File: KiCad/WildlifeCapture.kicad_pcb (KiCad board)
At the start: 2 copper layers, 105 x 100 mm, 15 parts, among them P1 USB_A, P2 GPS, SW1 A, SW2 LEADSW, U1 IM920_interplan, U3 STM32F103C8T6MinimumDevelopBo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, U4 RASPBERRYPI_GPIO_40

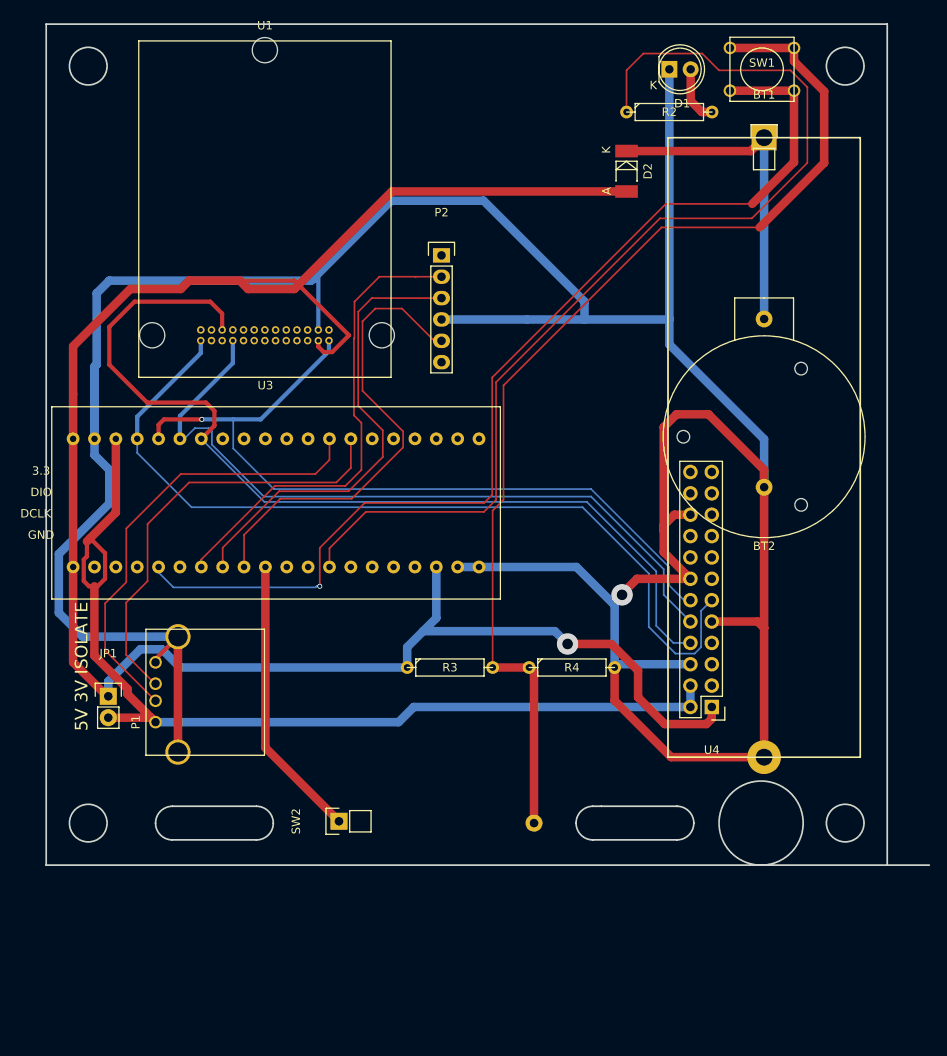
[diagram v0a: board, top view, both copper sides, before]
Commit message: Change to Take 2
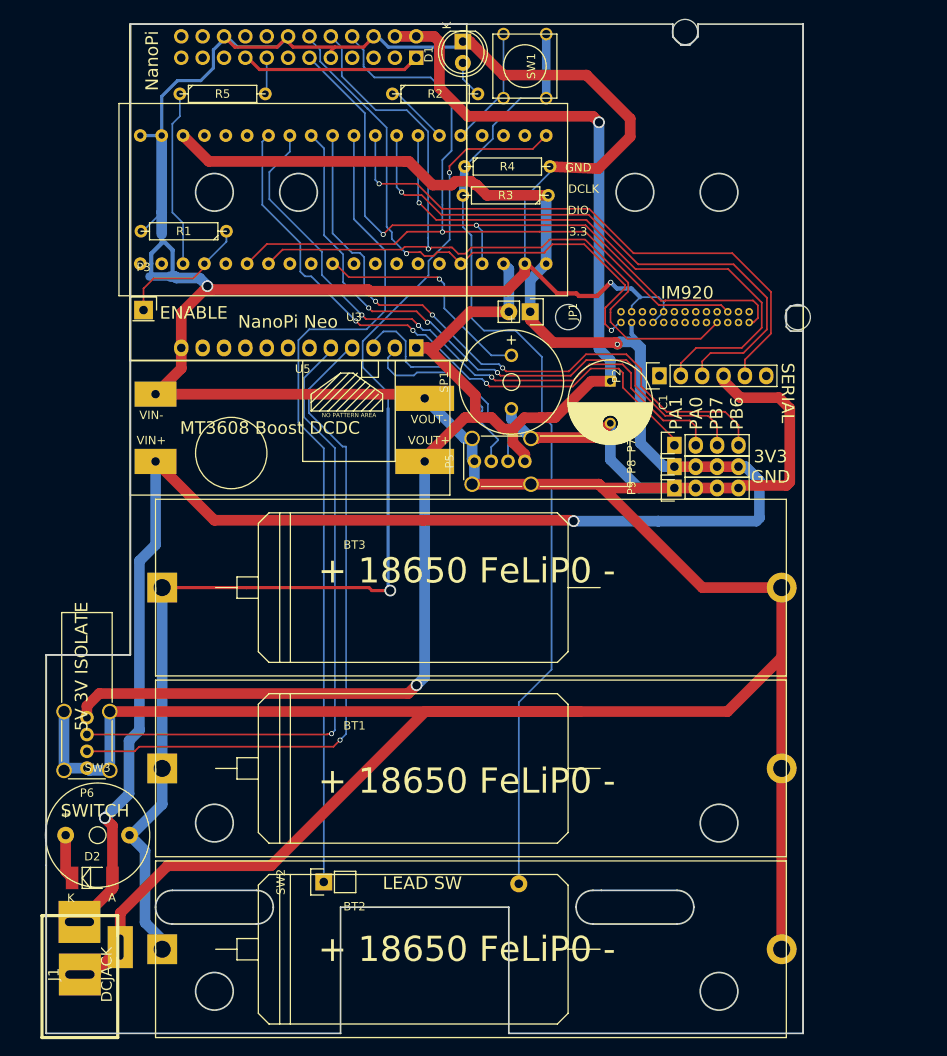
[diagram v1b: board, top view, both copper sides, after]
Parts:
- removed P1: USB_A, Connect:USB_A
- added BT3: Battery, library:18650BatteryCase, F.Cu at (134.1, 103.2)
- added C1: CP1, Capacitors_ThroughHole:C_Radial_D10_L13_P5, F.Cu at (158.2, 78.7)
- added J1: DCJACK, library:DCJACK, F.Cu at (95.1, 149.2)
- added P3: EN, Pin_Headers:Pin_Header_Straight_1x01, F.Cu at (102.7, 70.2)
- added P4: NanoPi_USB/Audio/IR, Pin_Headers:Pin_Header_Straight_1x12, B.Cu at (135.1, 74.7)
- added P5: USB_A, Connect:USB_A_Vertical, F.Cu at (148.0, 88.2)
- added P6: USB_A, Connect:USB_A_Vertical, F.Cu at (95.9, 118.7)
- added P7: SERVICE, Pin_Headers:Pin_Header_Straight_1x04, F.Cu at (165.8, 86.3)
- added P8: VCC, Pin_Headers:Pin_Header_Straight_1x04, F.Cu at (165.8, 88.9)
- added P9: GND, Pin_Headers:Pin_Header_Straight_1x04, F.Cu at (165.8, 91.4)
- added R1: R, Discret:R4, F.Cu at (107.4, 60.9)
- added R5: R, Discret:R4, F.Cu at (112.1, 44.5)
- added SP1: SPEAKER, Buzzers_Beepers:MagneticBuzzer_ProSignal_ABT-410-RC, F.Cu at (146.4, 82.0)
- added SW3: SWITCH_INV, Buzzers_Beepers:Buzzer_12x9.5RM7.6, F.Cu at (97.2, 132.7)
- added U5: MT3608, library:MT3608, F.Cu at (120.1, 84.2)
- BT1: footprint Pin_Headers:Pin_Header_Straight_1x02 -> library:18650BatteryCase
- BT2: footprint library:BATTERY_CR2032_CH25-2032LF_CONFORTABLE -> library:18650BatteryCase
- U1, U4: moved to B.Cu
- moved D2 105.3 mm to (96.6, 137.8), turned to 0 degrees
- moved BT1 86.1 mm to (134.1, 124.7)
- moved U4 84.8 mm to (135.1, 40.2), turned to 90 degrees
- moved BT2 74.2 mm to (134.1, 146.2), turned to 0 degrees
- moved JP1 67.9 mm to (148.6, 70.4), turned to 270 degrees
- moved R4 60.1 mm to (145.9, 53.2)
- moved R3 56.5 mm to (145.7, 56.6), turned to 180 degrees
- moved U1 50.0 mm to (167.0, 71.1), turned to 180 degrees
- moved U3 47.2 mm to (99.7, 68.5), turned to 0 degrees
- moved P2 29.6 mm to (164.0, 78.1), turned to 90 degrees
- moved SW1 28.2 mm to (148.0, 41.2), turned to 270 degrees
- moved R2 27.9 mm to (137.3, 44.5)
- moved D1 24.8 mm to (140.6, 38.3), turned to 270 degrees
- moved SW2 7.44 mm to (124.1, 138.2)
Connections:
- net Net-(JP1-Pad2) renamed +5V
- D2 pad 1: Net-(BT1-Pad1) -> Net-(D2-Pad1)
- D2 pad 2: +3V3 -> +BATT
- JP1 pad 1: +3V3 -> +BATT
- R3 pad 1: +3V3 -> +BATT
- U1 pad 18: Net-(U1-Pad18) -> GND
- U1 pad 19: Net-(U1-Pad19) -> GND
- U1 pad 23: +3V3 -> +BATT
- U3 pad 14: Net-(U1-Pad6) -> Net-(U3-Pad14)
- U3 pad 15: Net-(U1-Pad7) -> Net-(U3-Pad15)
- U3 pad 20: +3V3 -> +BATT
- U3 pad 21: +3V3 -> Net-(BT1-Pad1)
- U3 pad 26: Net-(U3-Pad26) -> Net-(R2-Pad1)
- U3 pad 33: Net-(R2-Pad1) -> Net-(P7-Pad2)
- U3 pad 38: +3V3 -> +BATT
- U3 pad 6: Net-(U3-Pad6) -> Net-(U1-Pad6)
- U3 pad 7: Net-(P1-Pad3) -> Net-(U1-Pad7)
- U4 pad 17: Net-(U4-Pad17) -> +3V3
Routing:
- net +BATT: track 0.00 -> 263.7 mm, vias 0 -> 3
- net +3V3: track 249.8 -> 21.5 mm, vias 1 -> 0
- net GND: track 394.9 -> 601.9 mm, vias 1 -> 2
- net Net-(R2-Pad1): track 124.2 -> 7.64 mm
- net Net-(SW1-Pad2): track 124.8 -> 14.5 mm, vias 1 -> 0
- net Net-(BT1-Pad1): track 38.6 -> 142.7 mm, vias 0 -> 2
- net Net-(P4-Pad4): track 0.00 -> 81.9 mm, vias 0 -> 1
- net Net-(P4-Pad5): track 0.00 -> 78.7 mm, vias 0 -> 1
- net Net-(P7-Pad2): track 0.00 -> 77.0 mm, vias 0 -> 3
- net Net-(P7-Pad4): track 0.00 -> 76.9 mm, vias 0 -> 3
- net Net-(P7-Pad3): track 0.00 -> 75.7 mm, vias 0 -> 3
- net +5V: track 119.1 -> 194.3 mm, vias 0 -> 2
- net Net-(P7-Pad1): track 0.00 -> 74.6 mm, vias 0 -> 3
- net Net-(SW2-Pad1): track 33.9 -> 99.8 mm
- net Net-(U3-Pad8): track 54.1 -> 0.00 mm
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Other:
- board size 105 x 100 mm -> 90 x 120 mm
- board text added: "+ 18650 FeLiP0 -"
- board text added: "3V3 GND"
- board text added: "ENABLE"
- board text added: "IM920"
- board text added: "LEAD SW"
- board text added: "MT3608 Boost DCDC"
- board text added: "NanoPi"
- board text added: "NanoPi Neo"
- board text added: "PA1 PA0 PB7 PB6"
- board text added: "SERIAL"
- board text added: "SWITCH"
